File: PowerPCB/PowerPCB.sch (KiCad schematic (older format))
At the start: 21 parts, among them J1 Conn_01x03_Male, J2 Conn_01x08_Male, J3 STM Inputs, J4 STM Outputs, J5 Conn_01x07_Male, K1 HF3-06, U1 NCP1117-3.3_SOT223

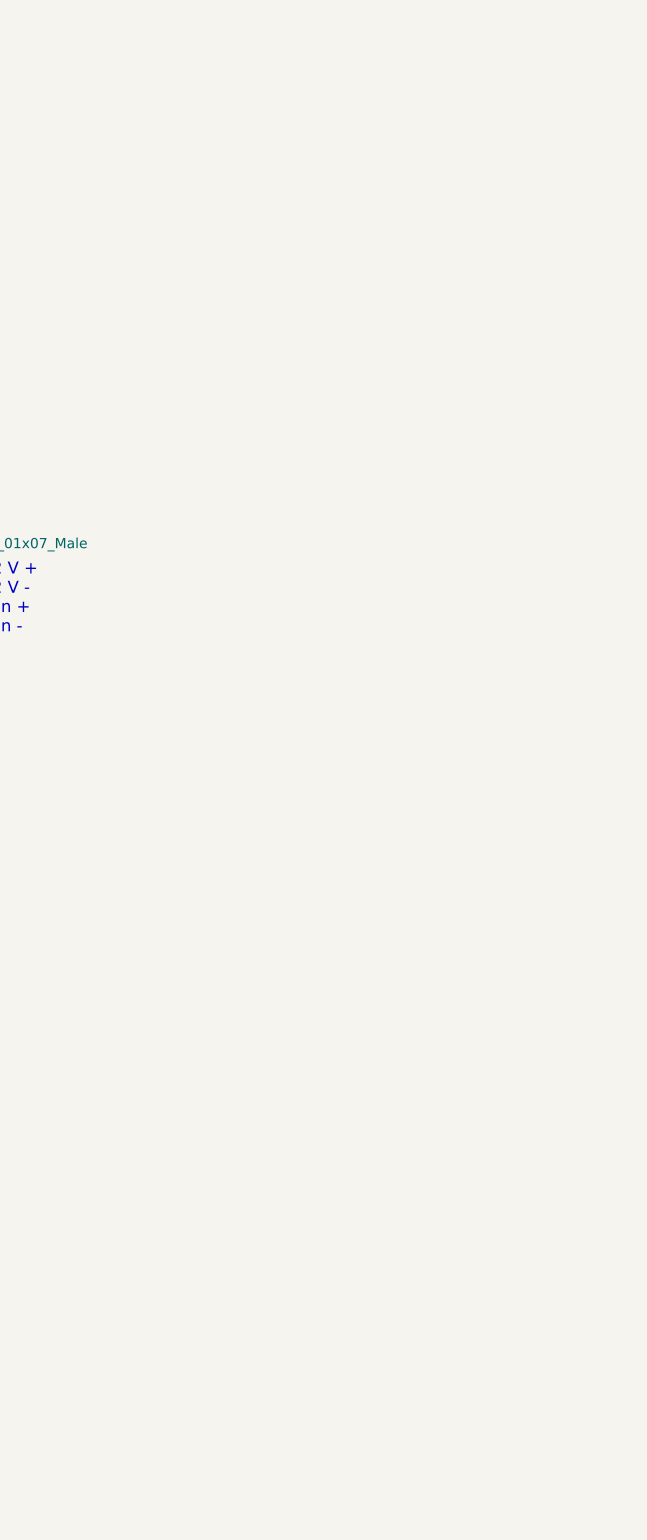
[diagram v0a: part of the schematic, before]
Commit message: Imported components to PCBnew
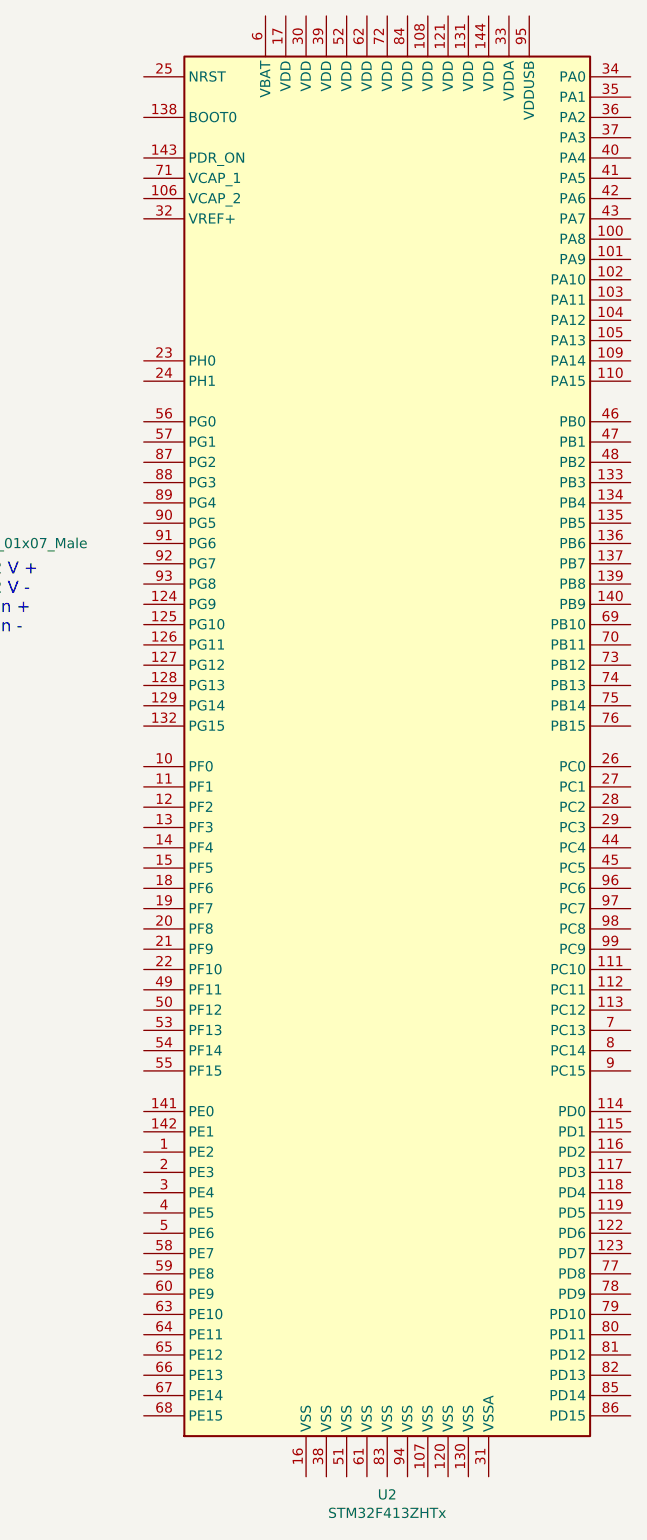
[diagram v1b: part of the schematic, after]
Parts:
- added U2: STM32F413ZHTx, Package_QFP:LQFP-144_20x20mm_P0.5mm, symbol MCU_ST_STM32F4:STM32F413ZHTx
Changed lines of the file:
@@
 Wire Wire Line
 	7800 3500 7950 3500
+$Comp
+L MCU_ST_STM32F4:STM32F413ZHTx U2
+U 1 1 5ECD68BB
+P 10200 4100
+F 0 "U2" H 10200 411 50  0000 C CNN
+F 1 "STM32F413ZHTx" H 10200 320 50  0000 C CNN
+F 2 "Package_QFP:LQFP-144_20x20mm_P0.5mm" H 9200 700 50  0001 R CNN
+F 3 "http://www.st.com/st-web-ui/static/active/en/resource/technical/document/datasheet/DM00282249.pdf" H 10200 4100 50  0001 C CNN
+	1    10200 4100
+	1    0    0    -1
+$EndComp
 $EndSCHEMATC
